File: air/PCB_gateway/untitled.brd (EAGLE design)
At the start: 109 x 66 mm, 16 parts, among them K1 351, Q1 S9013, U1 ESP32-DEVKITC-32D, U2 PC817X2NIP0F, X1 MSTBA2, X2 MSTBA2

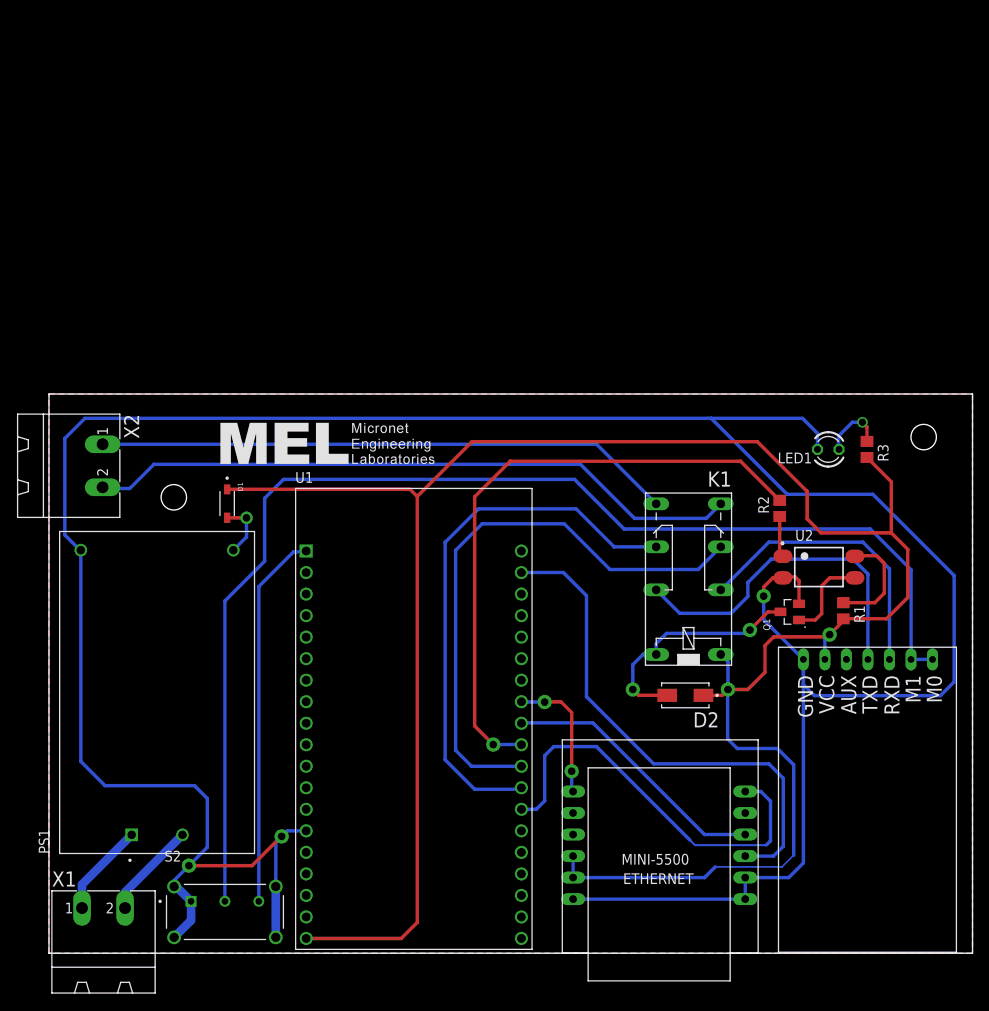
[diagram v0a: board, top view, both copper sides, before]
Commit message: revisi PCB dan List komponen
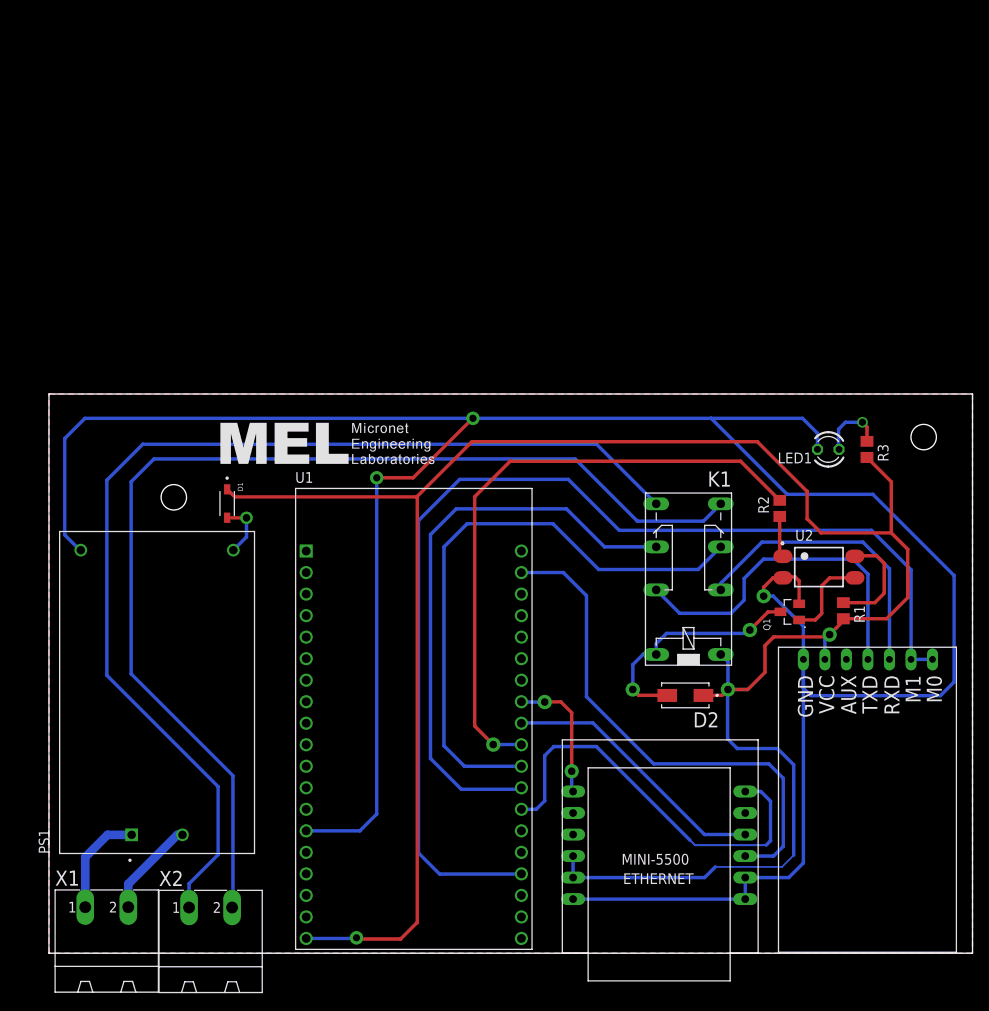
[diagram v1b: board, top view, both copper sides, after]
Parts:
- removed S2: EG1224, EG1224:SW_EG1224
- moved X2 59.9 mm to (19.1, 0.31), turned to 0 degrees
- moved X1 0.39 mm to (6.82, 0.35)
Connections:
- net 3V3: no longer S2.3
- net GND: no longer S2.1, S2.S1, S2.S2, S2.S3, S2.S4
- net M0: now also U1.35; no longer S2.2
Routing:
- net TXLORA_CONFIG: track 68.3 -> 126.8 mm
- net RXLORA_CONFIG: track 77.6 -> 129.9 mm
- net 3V3: track 44.5 -> 0.00 mm
- net GND: track 339.2 -> 314.1 mm
- net M0: track 144.3 -> 130.1 mm
- net TXLORA_MICRO: track 64.6 -> 68.5 mm
- net RXLORA_MICRO: track 68.1 -> 70.8 mm
- net N$1: track 11.1 -> 12.5 mm
- net TX_LORA: track 40.5 -> 41.1 mm
- net VCC: track 264.3 -> 264.5 mm, vias 2 -> 3

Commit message: revisi tanggal 24/02/2023
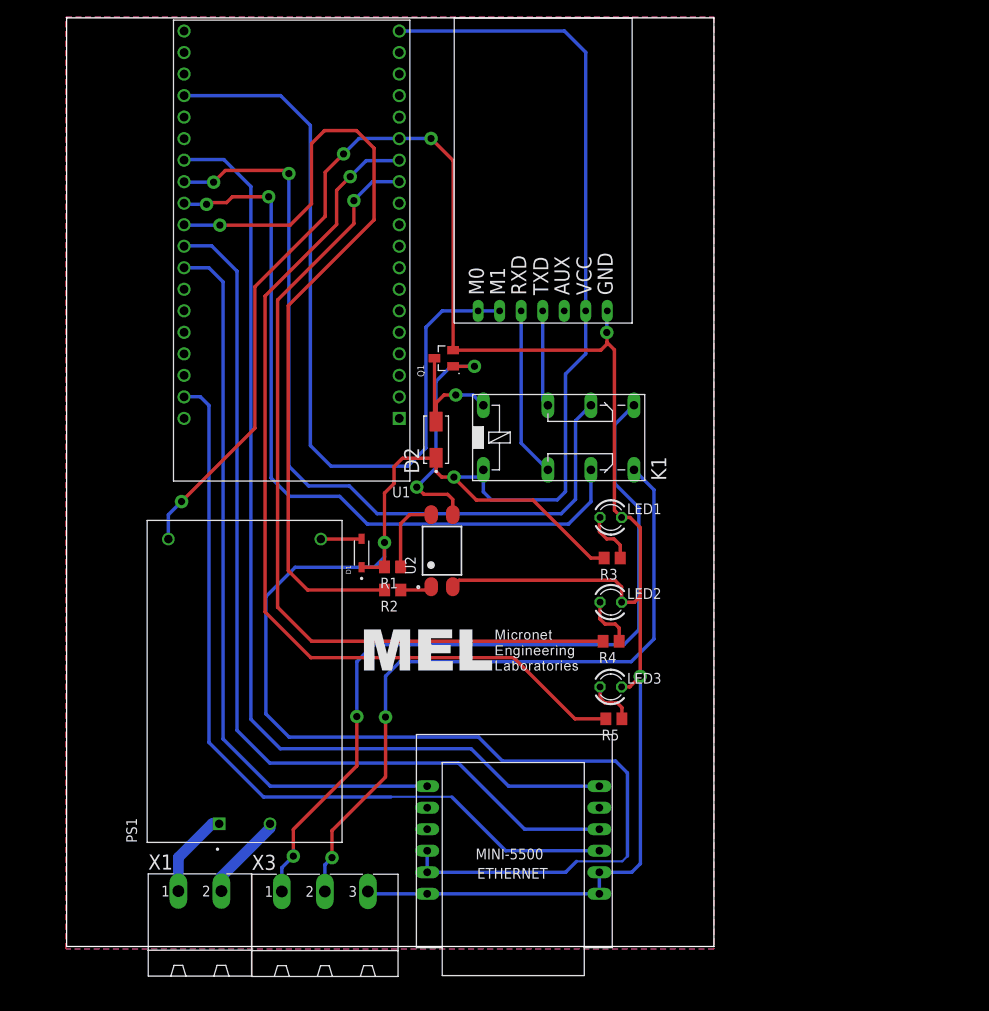
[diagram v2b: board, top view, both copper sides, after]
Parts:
- removed X2: MSTBA2, con-phoenix-508:MSTBA2
- added LED2, LED3: TLLY4400, led:LED3MM
- added R4, R5: (no value), rcl:R0805
- added X3: MSTBA3, con-phoenix-508:MSTBA3
- moved EBYTEE220-900T22D1 74.7 mm to (49.8, 80.4), turned to 90 degrees
- moved U1 57.0 mm to (28.6, 82.9), turned to 180 degrees
- moved R1 53.5 mm to (40.6, 45.6), turned to 180 degrees
- moved Q1 50.6 mm to (46.6, 70.2)
- moved R2 46.7 mm to (40.6, 42.9), turned to 180 degrees
- moved U2 44.5 mm to (46.4, 47.5), turned to 90 degrees
- moved D2 42.1 mm to (45.7, 60.6), turned to 90 degrees
- moved R3 32.7 mm to (66.5, 46.6), turned to 180 degrees
- moved K1 29.9 mm to (55.1, 60.9), turned to 0 degrees
- moved LED1 26.9 mm to (66.3, 51.4), turned to 0 degrees
- moved U$1 17.2 mm to (66.5, 0.66)
- moved D1 16.9 mm to (36.9, 47.2), turned to 90 degrees
- moved X1 11.2 mm to (17.8, 2.25)
- moved PS1 10.4 mm to (23.1, 32.1)
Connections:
- new net LED_PRS: R4.2, U1.12
- new net LED_WRN: R5.2, U1.13
- new net N$11: LED3.A, R5.1
- new net N$9: LED2.A, R4.1
- net GND: now also LED2.K, LED3.K, X3.3
- net RXLORA_CONFIG: now also X3.2; no longer X2.2
- net TXLORA_CONFIG: now also X3.1; no longer X2.1
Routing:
- net LED_WRN: track 0.00 -> 107.6 mm, vias 0 -> 1
- net LED_PRS: track 0.00 -> 98.1 mm, vias 0 -> 1
- net SCK_VSPI: track 31.9 -> 109.3 mm
- net GND: track 314.1 -> 240.2 mm, vias 3 -> 5
- net MISO_VSPI: track 15.9 -> 85.6 mm, vias 2 -> 0
- net INT_LAN: track 48.8 -> 116.5 mm
- net RXLORA_CONFIG: track 129.9 -> 82.9 mm, vias 0 -> 2
- net M0: track 130.1 -> 93.4 mm
- net MOSI_VSPI: track 60.9 -> 94.5 mm
- net TXLORA_CONFIG: track 126.8 -> 94.2 mm, vias 0 -> 2
- net TX_LORA: track 41.1 -> 11.4 mm
- net TXLORA_MICRO: track 68.5 -> 96.4 mm, vias 0 -> 2
- net CONFIG_LORA: track 73.1 -> 98.5 mm
- net RXLORA_MICRO: track 70.8 -> 88.6 mm, vias 0 -> 2
- net N$7: track 10.6 -> 27.9 mm, vias 0 -> 2
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- added copper zone on layer 1, net N$12
- added copper zone on layer 16, net N$5
- removed copper zone on layer 1, net N$5
- removed copper zone on layer 16, net N$9
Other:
- board size 109 x 66 mm -> 76.4 x 109.6 mm
